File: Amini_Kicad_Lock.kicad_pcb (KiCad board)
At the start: 2 copper layers, 29 x 20.1 mm, 45 parts, among them J1 Conn_01x02, J2 Conn_01x04, J3 MM8130-2600RA2, U1 nRF5340-QKxx, X1 32MHz, X2 32.768kHz

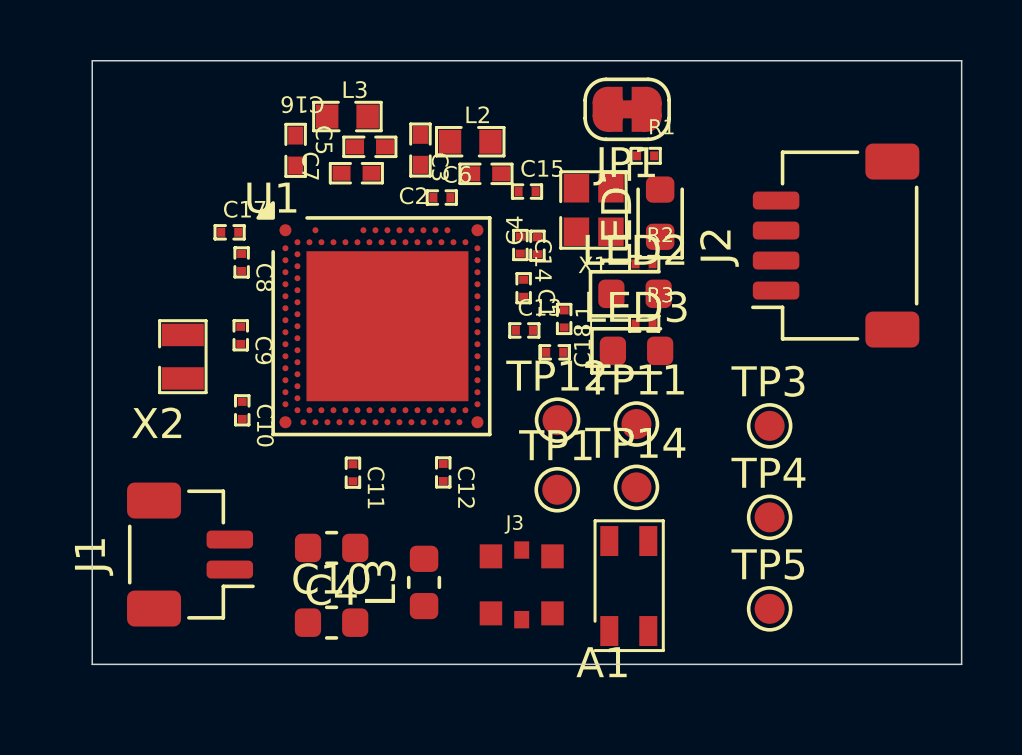
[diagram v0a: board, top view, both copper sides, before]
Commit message: clear, every component on place, component match kicad
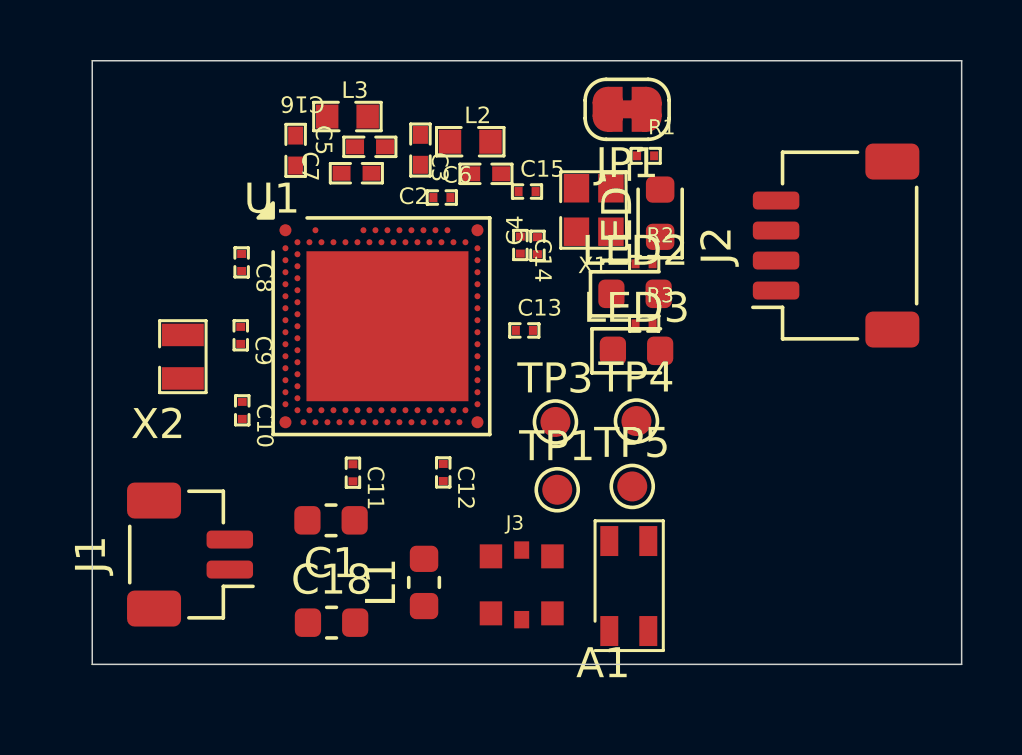
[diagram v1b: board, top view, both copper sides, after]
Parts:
- removed the C1 at (181.9, 60.4)
- removed C17: 100nF, Nordic_Semiconductor:CAPC0603X03L_C
- removed the C18 at (184.4, 62.5)
- removed the L1 at (184.5, 61.6)
- removed TP11, TP12, TP14: TestPoint, TestPoint:TestPoint_Pad_D1.0mm
- C1: renamed from C4; value 2.2nF -> 0.7pF
- C18: renamed from C10; value 100nF -> N.C.
- L1: renamed from L3; value 10µH -> 2.2nH
- moved TP3 7.14 mm to (183.0, 65.0)
- moved TP5 6.13 mm to (185.6, 67.2)
- moved TP4 5.48 mm to (185.7, 65.0)
- moved C1 0.92 mm to (175.5, 68.3)
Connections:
- C1 pad 1: Net-(U1-DECR) -> GND
- C1 pad 2: GND -> Net-(U1-ANT)
- C18 pad 1: VDD_nRF -> GND
- C18 pad 2: GND -> Net-(C18-Pad2)
- L1 pad 1: Net-(U1-DECD) -> Net-(U1-ANT)
- L1 pad 2: Net-(U1-DCCD) -> Net-(C18-Pad2)
